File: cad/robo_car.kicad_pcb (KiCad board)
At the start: 2 copper layers, 100 x 100 mm, 85 parts, among them J1 Conn_01x06_MountingPin, J16 Conn_01x02_MountingPin, J2 ftdi_conn, J3 Conn_01x06_MountingPin, J4 Conn_01x04, J5 Conn_01x04, J6 Conn_01x06_MountingPin, J7 Conn_01x02_MountingPin, J8 Conn_01x02_MountingPin, SW1 SW_Push, SW2 SW_Push, U1 XL1509, U2 AMS1117-3.3, U3 ESP32-WROOM-32U, U4 MOTOR_DRIVER-LV8548MC-AH, U5 Trans_CAN_SN65HVD230DR

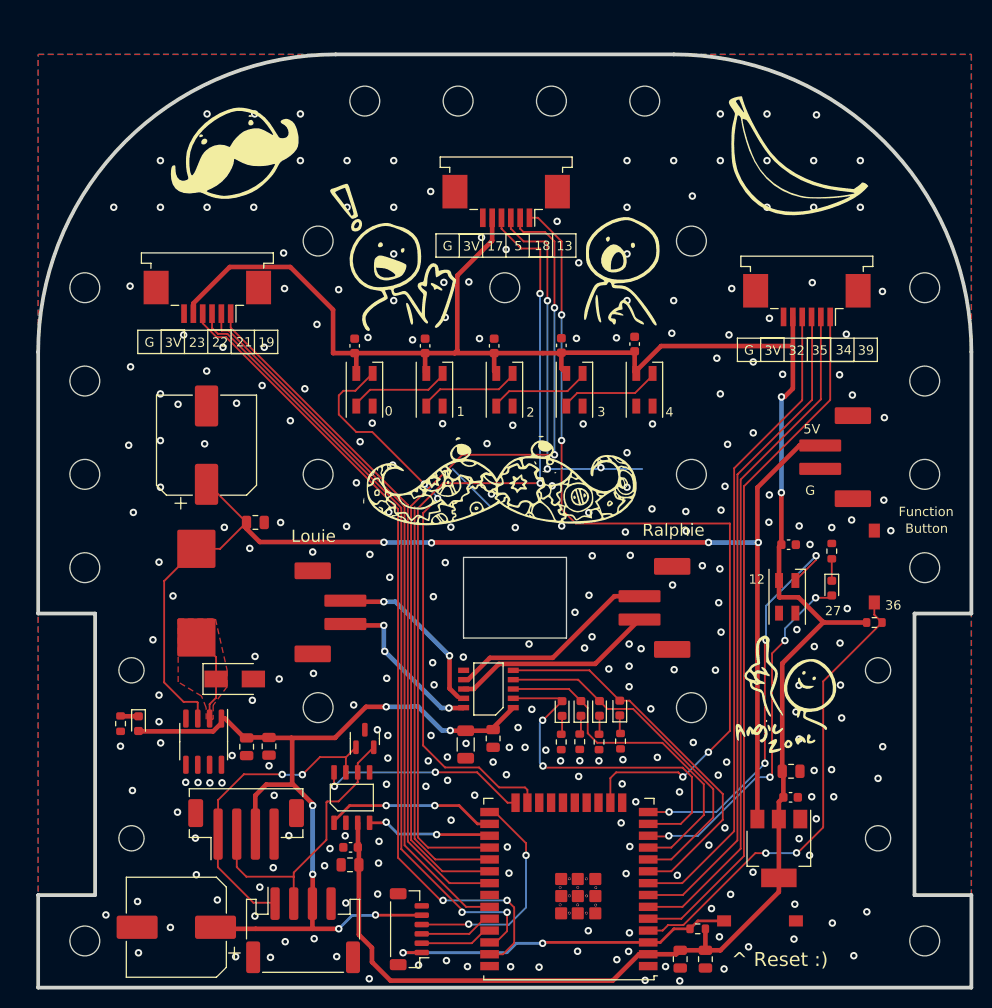
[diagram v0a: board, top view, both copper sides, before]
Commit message: Olivia Attempts Andrewism, and Abolishes Her Awesome Highway
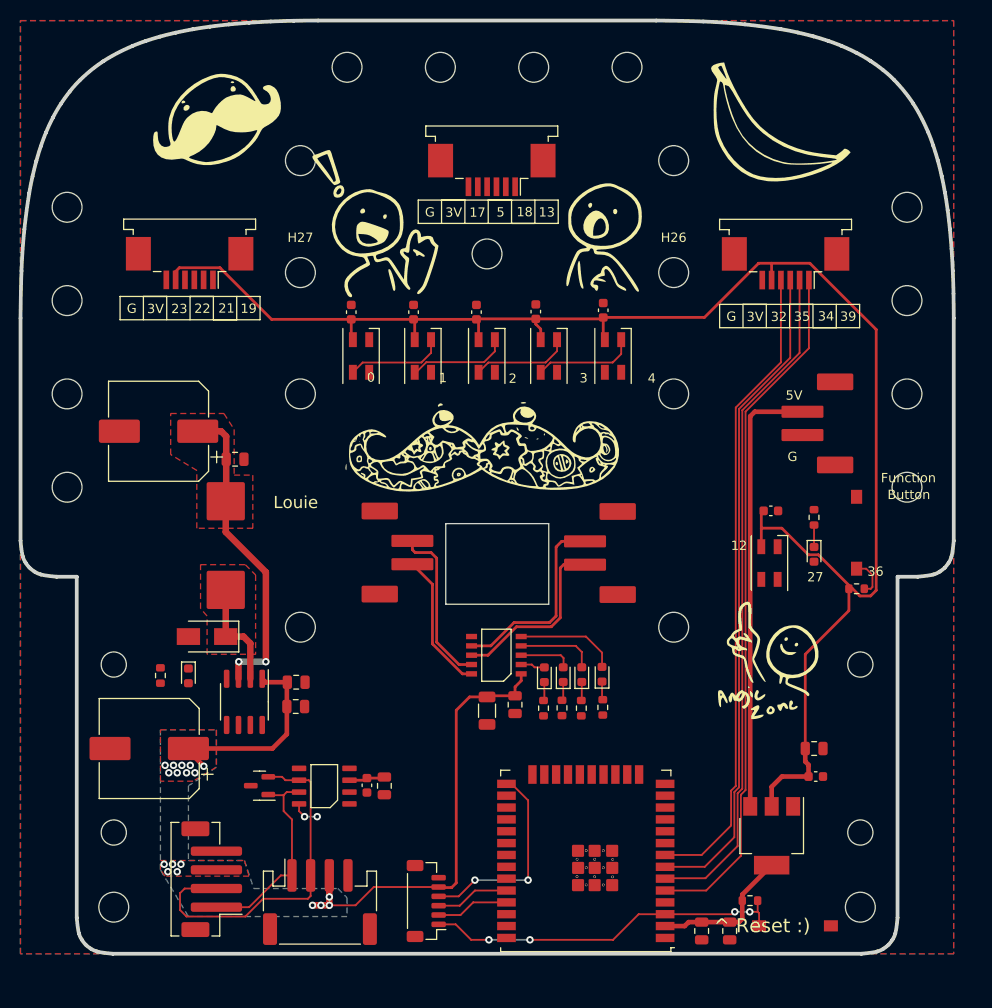
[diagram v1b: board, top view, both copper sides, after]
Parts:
- added H26: MountingHole, MountingHole:MountingHole_3.2mm_M3_ISO14580, F.Cu at (170.0, 77.0)
- added H27: MountingHole, MountingHole:MountingHole_3.2mm_M3_ISO14580, F.Cu at (130.0, 77.0)
- moved C1 19.4 mm to (113.8, 128.0)
- moved D7 12.4 mm to (125.6, 132.0), turned to 180 degrees
- moved J8 9.62 mm to (136.8, 107.0)
- moved C15 9.23 mm to (139.0, 132.0), turned to -90 degrees
- moved H1 8.83 mm to (130.0, 115.0)
- moved H11 8.83 mm to (130.0, 65.0)
- moved H12 8.83 mm to (105.0, 80.0)
- moved H13 8.83 mm to (105.0, 70.0)
- moved H15 8.83 mm to (195.0, 100.0)
- moved H17 8.83 mm to (105.0, 100.0)
- moved H18 8.83 mm to (195.0, 80.0)
- moved H20 8.83 mm to (195.0, 90.0)
- moved H25 8.83 mm to (195.0, 70.0)
- moved H3 8.83 mm to (170.0, 65.0)
- moved H5 8.83 mm to (105.0, 90.0)
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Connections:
- U3 pad 13: /MOTOR_L_1 -> /NEO_STATUS
- U3 pad 14: /NEO_STATUS -> /MOTOR_L_1
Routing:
- net /INPUT_D: track 92.0 -> 0.00 mm, vias 4 -> 0
- net /INPUT_B: track 91.5 -> 0.00 mm, vias 2 -> 0
- net /INPUT_A: track 90.3 -> 0.00 mm, vias 2 -> 0
- net /SDA: track 89.2 -> 0.00 mm, vias 2 -> 0
- net /INPUT_C: track 89.0 -> 0.00 mm, vias 2 -> 0
- net /SCL: track 85.1 -> 0.00 mm, vias 2 -> 0
- net /SERVO_0: track 77.4 -> 0.00 mm
- net /SERVO_1: track 75.0 -> 0.00 mm
- net /NEO_BAR: track 62.7 -> 0.00 mm, vias 2 -> 0
- net /VREG_OUT: track 134.8 -> 81.6 mm, vias 4 -> 2
- net +3V3: track 241.1 -> 193.2 mm, vias 2 -> 0
- net /FUNCTION_BUTTON: track 50.4 -> 4.23 mm, vias 2 -> 0
- net /NEO_STATUS: track 42.8 -> 0.00 mm, vias 4 -> 0
- net /HBT_LED: track 38.8 -> 0.00 mm, vias 4 -> 0
- net /MOTOR_L_1: track 38.9 -> 2.61 mm, vias 2 -> 0
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- added copper zone on F.Cu, net /VREG_OUT
- added copper zone on B.Cu, net VBUS
- added copper zone on F.Cu, net VBUS
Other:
- outline, holes or cut-outs redrawn
- board text removed: "Ralphie"
